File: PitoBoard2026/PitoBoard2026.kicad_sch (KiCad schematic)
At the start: 74 parts, among them J1 RJ25, J2 ICSP, J3 Conn_01x04_Socket, J4 Conn_01x04_Pin, SW1 RST, U1 ATmega328PB-A, U10 MCP25625-x-SS, U2 R-78E5.0-0.5, U3 MCP3425Axx-xCH, U4 SLIP, U7 SLIP, U8 R-78E3.3-0.5, U9 BME280, Y1 16MHz, Y3 16MHz

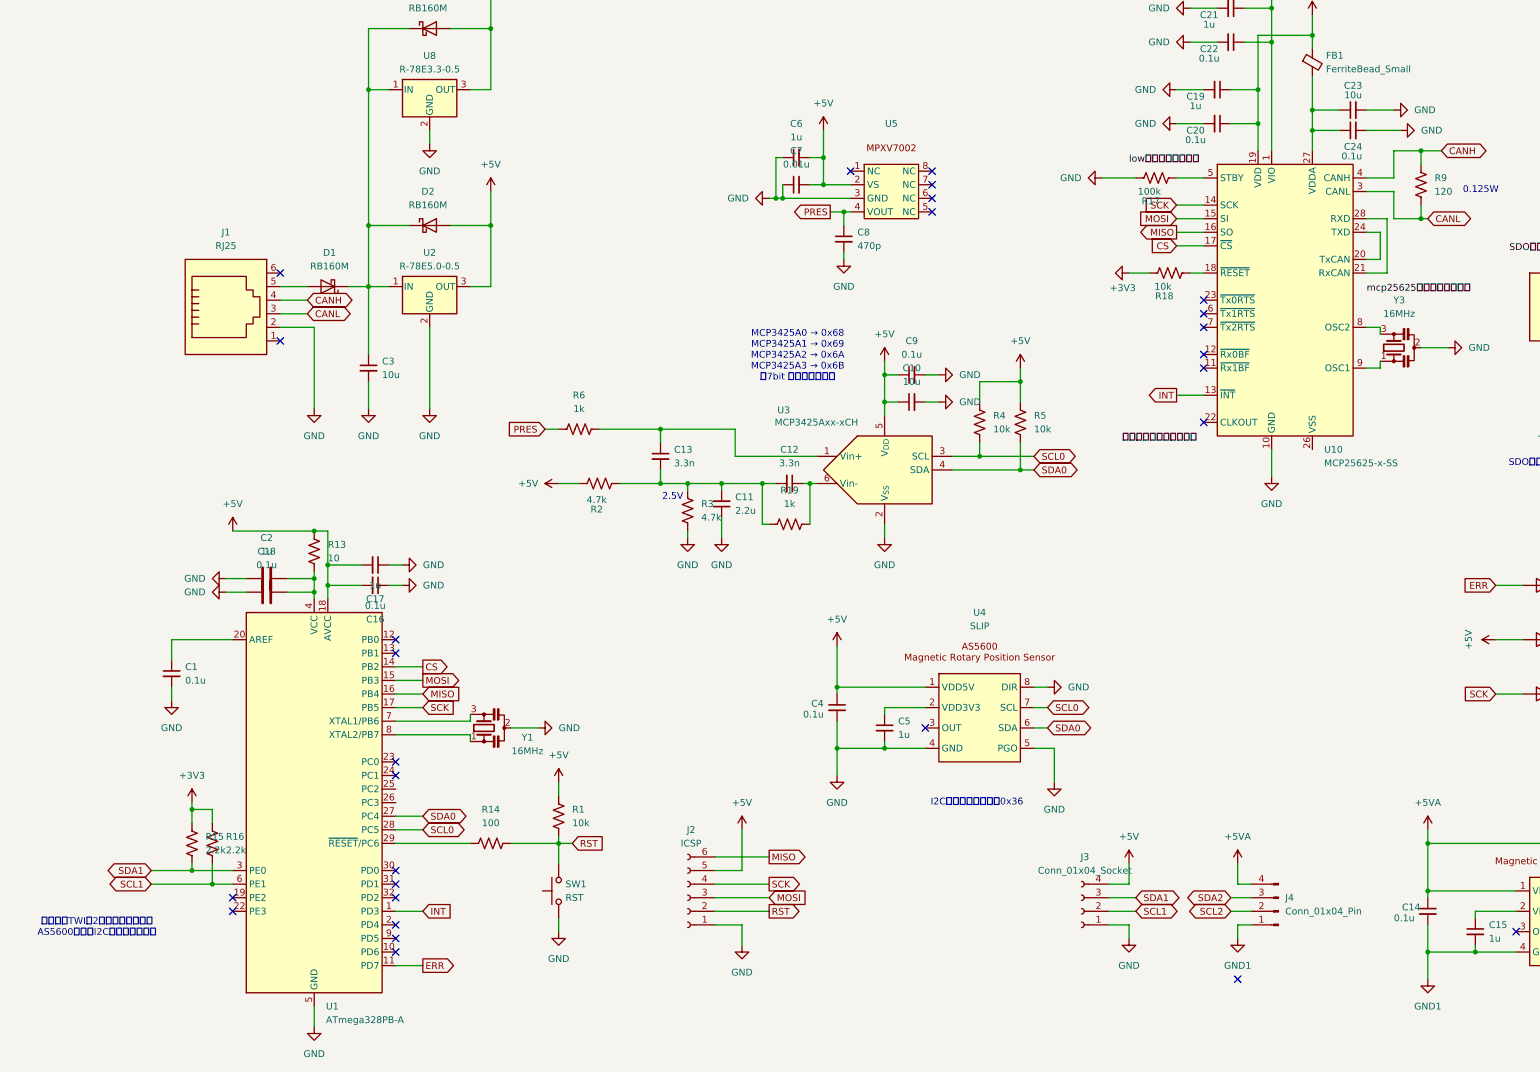
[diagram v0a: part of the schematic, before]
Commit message: Add files via upload
SDP32を配置
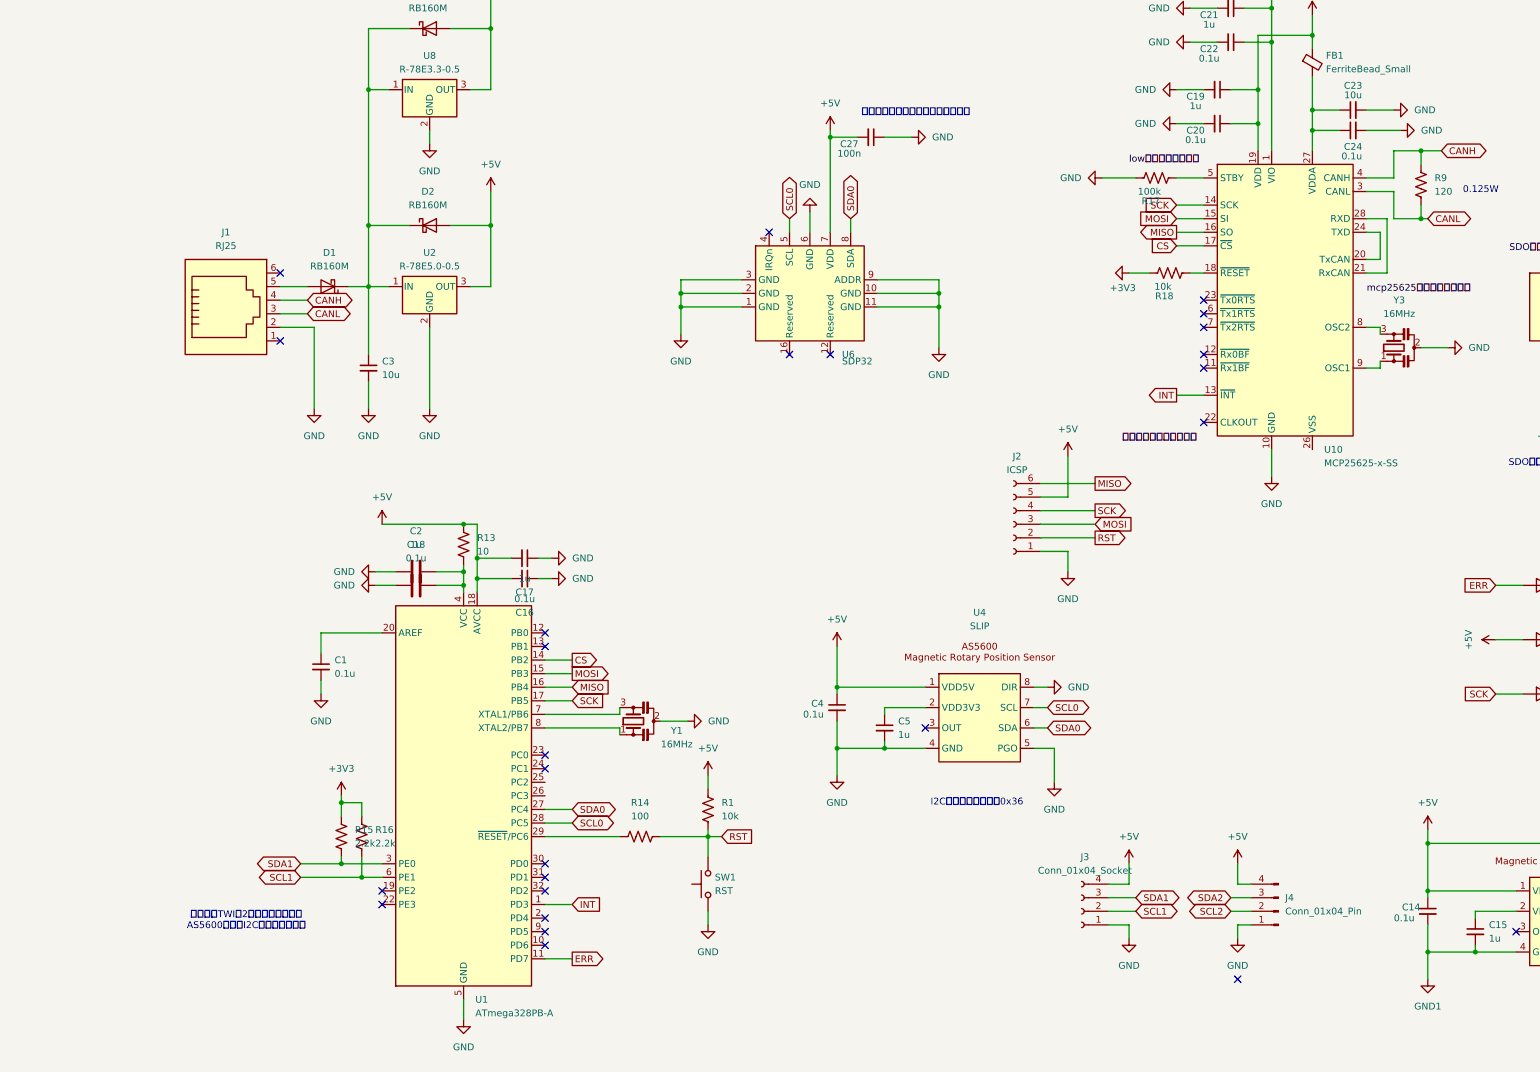
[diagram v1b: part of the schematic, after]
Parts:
- removed C10: 10u, Capacitor_SMD:C_1206_3216Metric, symbol Device:C_Small
- removed C11: 2.2u, Capacitor_SMD:C_1206_3216Metric, symbol Device:C_Small
- removed C12, C13: 3.3n, Capacitor_SMD:C_1206_3216Metric, symbol Device:C_Small
- removed C6: 1u, Capacitor_SMD:C_0805_2012Metric, symbol Device:C_Small
- removed C7: 0.01u, Capacitor_SMD:C_0603_1608Metric, symbol Device:C_Small
- removed C8: 470p, Capacitor_SMD:C_0603_1608Metric, symbol Device:C_Small
- removed C9: 0.1u, Capacitor_SMD:C_0603_1608Metric, symbol Device:C_Small
- removed R19, R6: 1k, Resistor_SMD:R_0603_1608Metric, symbol Device:R_US
- removed R2, R3: 4.7k, Resistor_SMD:R_0603_1608Metric, symbol Device:R_US
- removed R4, R5: 10k, Resistor_SMD:R_0603_1608Metric, symbol Device:R_US
- removed U3: MCP3425Axx-xCH, Package_TO_SOT_SMD:SOT-23-6, symbol Analog_ADC:MCP3425Axx-xCH
- removed U5: ~, KUBTSS_parts:MPXV7002, symbol KUBTSS_parts:MPXV7002
- added C27: 100n, Capacitor_SMD:C_0603_1608Metric, symbol Device:C_Small
- added U6: SDP32, symbol KUBTSS:SDP32
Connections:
- net +5VA is gone; now on net +5V: C14.1, J4.4 (Pin_4), R11.1, R12.1, U7.1 (VDD5V)
- net +5V: now also C27.2, U6.7 (VDD)
- net GND: now also J4.1 (Pin_1), C27.1, U6.1 (GND), U6.10 (GND), U6.11 (GND), U6.2 (GND), U6.3 (GND), U6.6 (GND), U6.9 (ADDR)
- net GND1: no longer J4.1 (Pin_1)
- net SCL0: now also U6.5 (SCL)
- net SDA0: now also U6.8 (SDA)
- no-connect marks 28 -> 26
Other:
- note added: "できるだけピンの近くに配置する。"
- note removed: "2.5V"
- note removed: "MCP3425A0 → 0x68 MCP3425A1 → 0x69 MCP3425A2 → 0x6A MCP3425A3 → 0x6B （7bit アドレス表記）"
- moved on the sheet: C1, C16, C17, C18, C2, J2, R1, R13, R14, R15, R16, SW1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

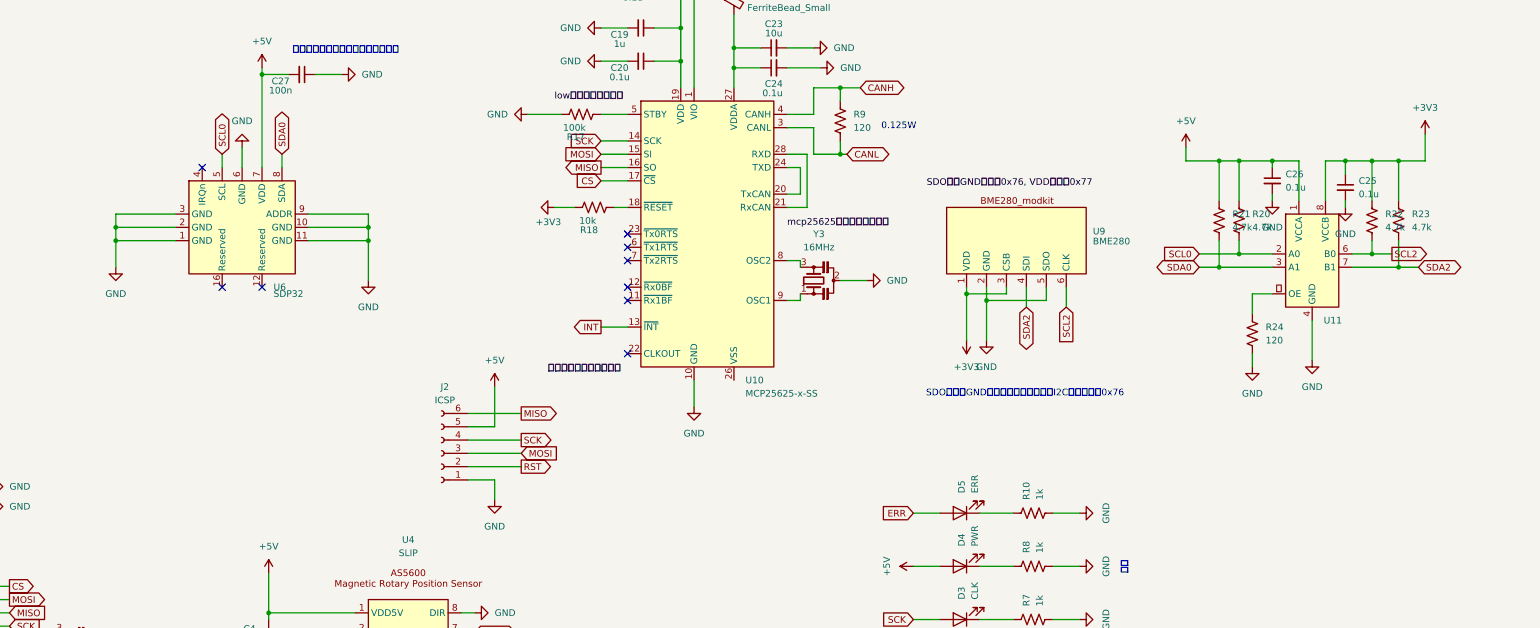
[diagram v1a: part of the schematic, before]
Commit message: Add files via upload
フットプリント設定完了
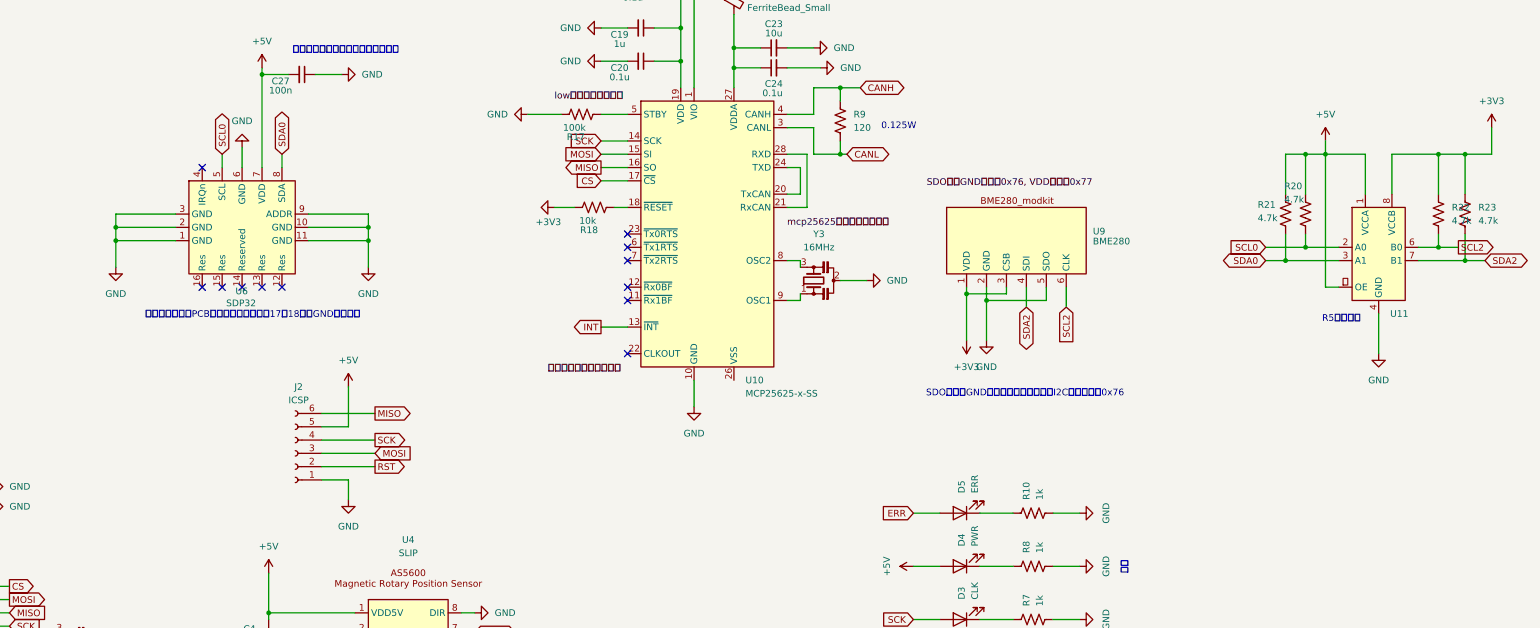
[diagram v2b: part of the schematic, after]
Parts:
- removed C25, C26: 0.1u, Capacitor_SMD:C_0805_2012Metric, symbol Device:C_Small
- removed R24: 120, Resistor_SMD:R_0603_1608Metric, symbol Device:R_US
- FB1: footprint (none) -> Inductor_SMD:L_0603_1608Metric
- U11: footprint (none) -> Package_DIP:DIP-8_W7.62mm
- U6: footprint (none) -> KUBTSS:SDP32
- U9: footprint KUBTSS_parts:Temp_AE-BME280 -> KUBTSS:BME280
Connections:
- net +5V: now also U11.５ (OE)
- no-connect marks 26 -> 29
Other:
- note added: "R5をはがす"
- note added: "裏面のパッド（PCBエディターでパッド17、18）はGNDにする。"
- moved on the sheet: J2, R20, R21, R22, R23, U11
